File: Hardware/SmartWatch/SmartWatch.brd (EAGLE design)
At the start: 36.8 x 40.6 mm, 91 parts, among them T1 TESTPOINT-0603, T2 TESTPOINT-0603, T3 TESTPOINT-0603, T4 TESTPOINT-0603, T5 TESTPOINT-0603, U1 STM32L476, U10 MICRO-USB, U11 BNO055, U12 MAX17048, U3 UG-2828GDEDF11, U4 FAN5331SX, U5 APDS-9960, U6 MCP73831, U7 AP2112K-3.3TRG-1, U8 ASDK-32.768, U9 ASCO-8

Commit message: updated bom
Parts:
- R23, R24, R25: value 10k -> 82
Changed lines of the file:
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@@
 <setting verticaltext="up"/>
 </settings>
-<grid distance="0.01" unitdist="inch" unit="inch" style="lines" multiple="1" display="yes" altdistance="0.001" altunitdist="inch" altunit="inch"/>
+<grid distance="0.05" unitdist="inch" unit="inch" style="lines" multiple="1" display="yes" altdistance="0.005" altunitdist="inch" altunit="inch"/>
 <layers>
 <layer number="1" name="Top" color="4" fill="1" visible="yes" active="yes"/>
@@
 <element name="D5" library="SparkFun-LED" package="LED-0603" value="" x="9.652" y="4.318" rot="R180"/>
 <element name="D6" library="SparkFun-LED" package="LED-0603" value="" x="11.176" y="4.318" rot="R180"/>
-<element name="R23" library="resistor" package="R0603" value="10k" x="8.128" y="7.493" rot="R270"/>
-<element name="R24" library="resistor" package="R0603" value="10k" x="9.652" y="7.493" rot="R270"/>
-<element name="R25" library="resistor" package="R0603" value="10k" x="11.176" y="7.493" rot="R270"/>
+<element name="R23" library="resistor" package="R0603" value="82" x="8.128" y="7.493" rot="R270"/>
+<element name="R24" library="resistor" package="R0603" value="82" x="9.652" y="7.493" rot="R270"/>
+<element name="R25" library="resistor" package="R0603" value="82" x="11.176" y="7.493" rot="R270"/>
 <element name="U12" library="SparkFun-DigitalIC" package="DFN-8" value="MAX17048" x="3.556" y="27.178" rot="R180">
 <attribute name="PROD_ID" value="IC-12551" x="7.366" y="20.828" size="1.778" layer="27" font="vector" ratio="15" rot="R180" display="off"/>

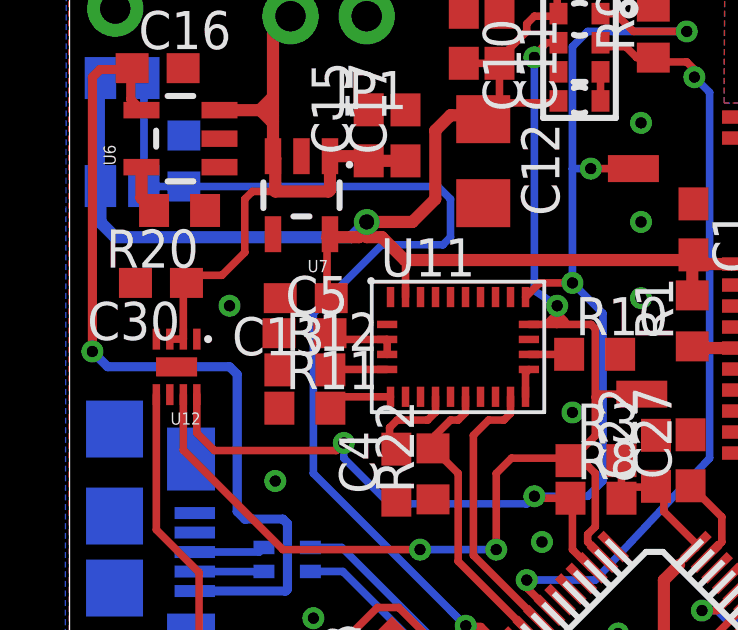
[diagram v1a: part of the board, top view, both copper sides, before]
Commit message: adding actual gerber files
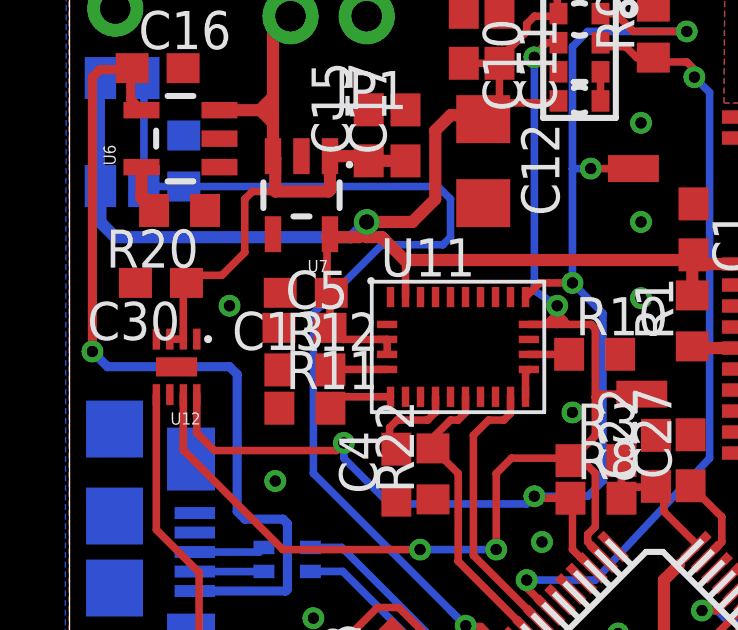
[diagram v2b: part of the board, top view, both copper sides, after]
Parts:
- moved C13 0.18 mm to (7.87, 29.6)
- moved C5 0.18 mm to (7.83, 28.5)
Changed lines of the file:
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@@
 <setting verticaltext="up"/>
 </settings>
-<grid distance="0.05" unitdist="inch" unit="inch" style="lines" multiple="1" display="yes" altdistance="0.005" altunitdist="inch" altunit="inch"/>
+<grid distance="0.01" unitdist="inch" unit="inch" style="lines" multiple="1" display="yes" altdistance="0.001" altunitdist="inch" altunit="inch"/>
 <layers>
 <layer number="1" name="Top" color="4" fill="1" visible="yes" active="yes"/>
@@
 </element>
 <element name="C4" library="resistor" package="C0603" value="0.1uF" x="10.894" y="23.58" rot="R90"/>
-<element name="C5" library="resistor" package="C0603" value="0.1uF" x="7.832" y="28.2954"/>
+<element name="C5" library="resistor" package="C0603" value="0.1uF" x="7.832" y="28.4732"/>
 <element name="C11" library="resistor" package="C0603" value="0.1uF" x="14.332" y="38.142" rot="R270"/>
 <element name="R9" library="resistor" package="R0603" value="10k" x="19.46" y="38.332" rot="R90"/>
@@
 <attribute name="PROD_ID" value="VREG-12457" x="11.542" y="26.546" size="1.778" layer="27" font="vector" ratio="15" rot="R180" display="off"/>
 </element>
-<element name="C13" library="resistor" package="C0603" value="2.2uF" x="7.874" y="29.464" rot="R180"/>
+<element name="C13" library="resistor" package="C0603" value="2.2uF" x="7.874" y="29.6418" rot="R180"/>
 <element name="C17" library="resistor" package="C0603" value="1uF" x="11.1986" y="34.8892" rot="R90">
 <attribute name="PROD_ID" value="CAP-00868" x="9.9286" y="27.2692" size="1.778" layer="27" font="vector" ratio="15" rot="R90" display="off"/>
@@
 <wire x1="11.2" y1="30.71" x2="11.176" y2="30.734" width="0.254" layer="1"/>
 <wire x1="10.5875" y1="28.088" x2="9.118" y2="28.088" width="0.254" layer="1"/>
-<wire x1="9.118" y1="28.088" x2="8.682" y2="28.2954" width="0.254" layer="1"/>
+<wire x1="9.118" y1="28.088" x2="8.682" y2="28.4732" width="0.254" layer="1"/>
 <wire x1="10.5875" y1="27.588" x2="10.5875" y2="28.088" width="0.254" layer="1"/>
-<wire x1="8.682" y1="28.2954" x2="8.682" y2="29.714621875" width="0.254" layer="1"/>
-<wire x1="8.682" y1="29.714621875" x2="8.724" y2="29.464" width="0.254" layer="1"/>
+<wire x1="8.682" y1="28.4732" x2="8.682" y2="29.714621875" width="0.254" layer="1"/>
+<wire x1="8.682" y1="29.714621875" x2="8.724" y2="29.6418" width="0.254" layer="1"/>
 <wire x1="9.906" y1="32.004" x2="11.43" y2="32.004" width="0.4064" layer="1"/>
 <wire x1="11.43" y1="32.004" x2="12.192" y2="32.766" width="0.4064" layer="1"/>
@@
 <wire x1="23.114" y1="5.322571875" x2="23.24410625" y2="5.452678125" width="0.254" layer="1"/>
 <wire x1="8.58380625" y1="31.49770625" x2="8.58380625" y2="29.939815625" width="0.254" layer="1"/>
-<wire x1="8.58380625" y1="29.939815625" x2="8.724" y2="29.464" width="0.254" layer="1"/>
+<wire x1="8.58380625" y1="29.939815625" x2="8.724" y2="29.6418" width="0.254" layer="1"/>
 <wire x1="18.77" y1="23.166" x2="19.7772" y2="23.166" width="0.254" layer="1"/>
 <wire x1="19.7772" y1="23.166" x2="19.5486" y2="23.1914" width="0.254" layer="1"/>
